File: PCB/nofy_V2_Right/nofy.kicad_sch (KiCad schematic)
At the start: 144 parts, among them J10 Conn_01x01-Connector_Generic, J11 Conn_01x01-Connector_Generic, J12 Conn_01x01-Connector_Generic, J13 Conn_01x01-Connector_Generic, J14 Conn_01x01-Connector_Generic, J15 Conn_01x01-Connector_Generic, J16 Conn_01x01-Connector_Generic, J17 Conn_01x01-Connector_Generic, J18 Conn_01x01-Connector_Generic, J19 Conn_01x01-Connector_Generic, J20 Conn_01x01-Connector_Generic, J21 Conn_01x01-Connector_Generic, J22 PIn1x4, J23 PIn1x4, J24 PIn1x4, J25 PIn1x4, J26 PIn1x4, J27 PIn1x4, J28 PIn1x4, J29 PIn1x4, J30 PIn1x4, J31 PIn1x4, J32 PIn1x4, J33 PIn1x4, J34 PIn1x4, J35 PIn1x4, J36 PIn1x4, J37 PIn1x4, J38 PIn1x4, J39 PIn1x4, J40 PIn1x4, J41 PIn1x4, SW1 RotaryEncoder, SW10 SW_PUSH, SW11 SW_PUSH, SW12 SW_PUSH, SW13 SW_PUSH, SW14 SW_PUSH, SW15 SW_PUSH, SW16 SW_PUSH, SW17 SW_PUSH, SW18 SW_PUSH, SW19 SW_PUSH, SW2 RotaryEncoder, SW20 SW_PUSH, SW21 SW_PUSH, SW22 SW_PUSH, SW23 SW_PUSH, SW24 SW_PUSH, SW25 SW_PUSH, SW26 SW_PUSH, SW27 SW_PUSH, SW28 SW_PUSH, SW29 SW_PUSH, SW3 SW_SPDT, SW30 SW_PUSH, SW31 SW_PUSH, SW32 SW_PUSH, SW33 SW_PUSH, SW34 SW_PUSH, SW35 SW_PUSH, SW36 SW_PUSH, SW37 SW_PUSH, SW38 SW_PUSH, SW39 SW_PUSH, SW4 SW_SPDT, SW40 SW_PUSH, SW41 SW_PUSH, SW42 SW_PUSH, SW43 SW_PUSH, SW44 SW_PUSH, SW45 SW_PUSH, SW46 SW_PUSH, SW47 SW_PUSH, SW48 SW_PUSH, SW49 SW_PUSH, SW5 SW_PUSH, SW50 SW_PUSH, SW51 SW_PUSH, SW52 SW_PUSH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

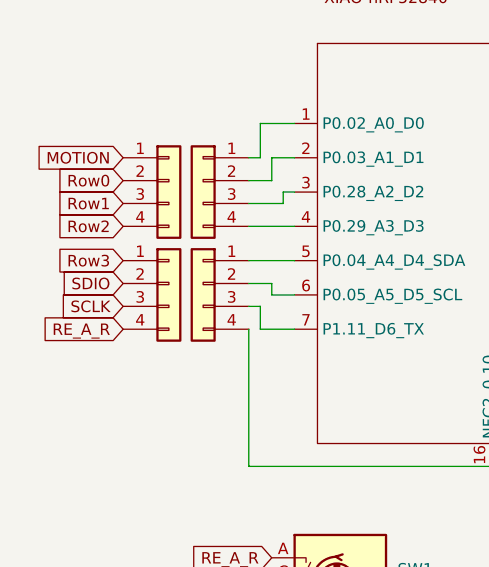
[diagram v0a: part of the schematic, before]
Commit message: pcb
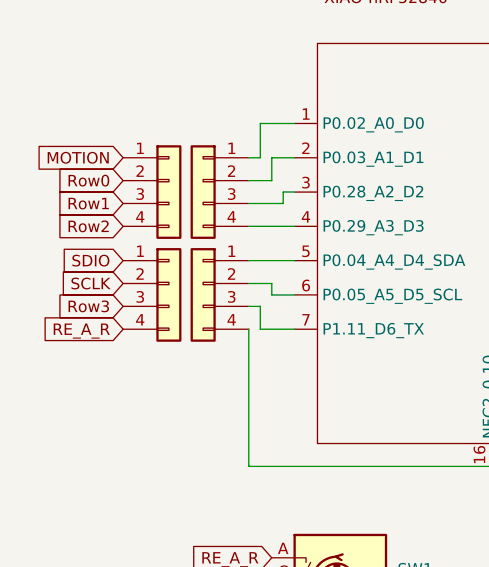
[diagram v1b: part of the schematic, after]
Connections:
- net Row3: now also J37.3 (Pin_3); no longer J37.1 (Pin_1)
- net SCLK: now also J37.2 (Pin_2); no longer J37.3 (Pin_3)
- net SDIO: now also J37.1 (Pin_1); no longer J37.2 (Pin_2)
